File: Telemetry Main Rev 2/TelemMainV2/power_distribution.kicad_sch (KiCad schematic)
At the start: 8 parts, among them U1 LM7805_TO220, U2 LM7809_TO220

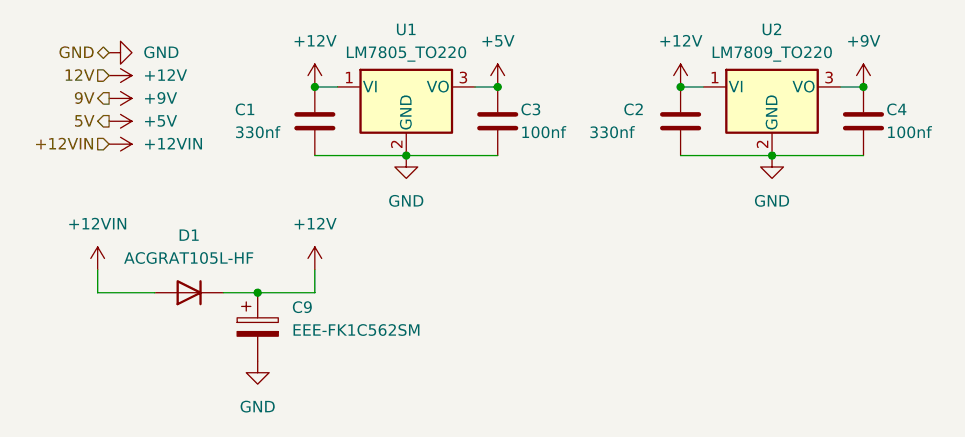
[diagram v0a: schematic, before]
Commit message: added status diodes, fixed silkscreen, etc
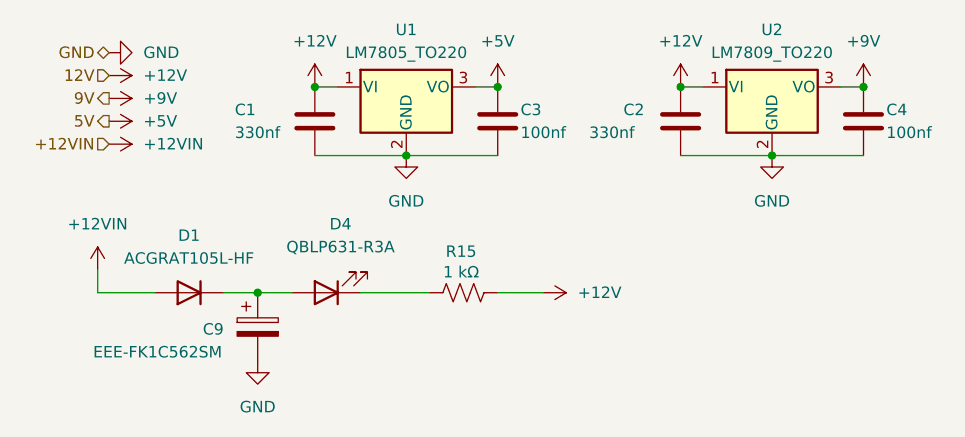
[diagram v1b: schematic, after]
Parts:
- added D4: QBLP631-R3A, LED_SMD:LED_0805_2012Metric_Pad1.15x1.40mm_HandSolder, symbol Device:LED
- added R15: 1 kΩ, Resistor_SMD:R_0805_2012Metric_Pad1.20x1.40mm_HandSolder, symbol Device:R_US
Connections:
- net +12V: now also R15.2; no longer C9.1, D1.1 (K)
- new net: D4.1 (K), R15.1
- new net: C9.1, D1.1 (K), D4.2 (A)
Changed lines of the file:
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@@
 	(wire
 		(pts
-			(xy 36.83 43.18) (xy 43.18 43.18)
+			(xy 36.83 43.18) (xy 40.64 43.18)
 		)
 		(stroke
@@
 	(wire
 		(pts
-			(xy 43.18 43.18) (xy 43.18 40.64)
+			(xy 48.26 43.18) (xy 55.88 43.18)
+		)
+		(stroke
+			(width 0)
+			(type default)
+		)
+	)
+	(wire
+		(pts
+			(xy 63.5 43.18) (xy 68.58 43.18)
 		)
 		(stroke
@@
 	)
 	(symbol
+		(lib_id "Device:LED")
+		(at 44.45 43.18 180)
+		(unit 1)
+		(exclude_from_sim no)
+		(in_bom yes)
+		(on_board yes)
+		(dnp no)
+		(fields_autoplaced yes)
+		(property "Reference" "D4"
+			(at 46.0375 35.56 0)
+			(effects
+				(font
+					(size 1.27 1.27)
+				)
+			)
+		)
+		(property "Value" "QBLP631-R3A"
+			(at 46.0375 38.1 0)
+			(effects
+				(font
+					(size 1.27 1.27)
+				)
+			)
+		)
+		(property "Footprint" "LED_SMD:LED_0805_2012Metric_Pad1.15x1.40mm_HandSolder"
+			(at 44.45 43.18 0)
+			(effects
+				(font
+					(size 1.27 1.27)
+				)
+				(hide yes)
+			)
+		)
+		(property "Datasheet" "https://www.qt-brightek.com/datasheet/QBLP631-R3A.pdf"
+			(at 44.45 43.18 0)
+			(effects
+				(font
+					(size 1.27 1.27)
+				)
+				(hide yes)
+			)
+		)
+		(property "Description" "12V Status LED"
+			(at 44.45 43.18 0)
+			(effects
+				(font
+					(size 1.27 1.27)
+				)
+				(hide yes)
+			)
+		)
+		(pin "1"
+		)
+		(pin "2"
+		)
+		(instances
+			(project "TelemMainV2"
+				(path "/dde73ecd-f7ea-407a-a1ab-cf1927044ecb/dcd9c4a0-8d80-4caa-a99a-0b76a5d913c0"
+					(reference "D4")
+					(unit 1)
+				)
+			)
+		)
+	)
+	(symbol
 		(lib_id "power:GND")
 		(at 20.32 16.51 90)
@@
 		(on_board yes)
 		(dnp no)
-		(fields_autoplaced yes)
 		(property "Reference" "C9"
-			(at 40.64 44.8309 0)
+			(at 30.734 47.244 0)
 			(effects
 				(font
@@
 		)
 		(property "Value" "EEE-FK1C562SM"
-			(at 40.64 47.3709 0)
+			(at 18.542 49.784 0)
 			(effects
 				(font
@@
 	(symbol
 		(lib_id "power:+12V")
-		(at 43.18 40.64 0)
+		(at 68.58 43.18 270)
 		(unit 1)
 		(exclude_from_sim no)
@@
 		(fields_autoplaced yes)
 		(property "Reference" "#PWR049"
-			(at 43.18 44.45 0)
+			(at 64.77 43.18 0)
 			(effects
 				(font
@@
 		)
 		(property "Value" "+12V"
-			(at 43.18 35.56 0)
-			(effects
-				(font
-					(size 1.27 1.27)
-				)
+			(at 72.39 43.1799 90)
+			(effects
+				(font
+					(size 1.27 1.27)
+				)
+				(justify left)
 			)
 		)
 		(property "Footprint" ""
-			(at 43.18 40.64 0)
+			(at 68.58 43.18 0)
 			(effects
 				(font
@@
 		)
 		(property "Datasheet" ""
-			(at 43.18 40.64 0)
+			(at 68.58 43.18 0)
 			(effects
 				(font
@@
 		)
 		(property "Description" "Power symbol creates a global label with name \"+12V\""
-			(at 43.18 40.64 0)
+			(at 68.58 43.18 0)
 			(effects
 				(font
@@
 					(unit 1)
 				)
+			)
+		)
+	)
+	(symbol
+		(lib_id "Device:R_US")
+		(at 59.69 43.18 90)
+		(unit 1)
+		(exclude_from_sim no)
+		(in_bom yes)
+		(on_board yes)
+		(dnp no)
+		(property "Reference" "R15"
+			(at 59.436 38.608 90)
+			(effects
+				(font
+					(size 1.27 1.27)
+				)
+			)
+		)
+		(property "Value" "1 kΩ"
+			(at 59.436 40.894 90)
+			(effects
+				(font
+					(size 1.27 1.27)
+				)
+			)
+		)
+		(property "Footprint" "Resistor_SMD:R_0805_2012Metric_Pad1.20x1.40mm_HandSolder"
+			(at 59.944 42.164 90)
+			(effects
+				(font
+					(size 1.27 1.27)
+				)
+				(hide yes)
+			)
+		)
+		(property "Datasheet" "~"
+			(at 59.69 43.18 0)
+			(effects
+				(font
+					(size 1.27 1.27)
+				)
+				(hide yes)
+			)
+		)
+		(property "Description" "Resistor, US symbol"
+			(at 59.69 43.18 0)
+			(effects
+				(font
+					(size 1.27 1.27)
+				)
+				(hide yes)
+			)
+		)
+		(pin "1"
+		)
+		(pin "2"
+		)
+		(instances
+			(project "TelemMainV2"
+				(path "/dde73ecd-f7ea-407a-a1ab-cf1927044ecb/dcd9c4a0-8d80-4caa-a99a-0b76a5d913c0"
+					(reference "R15")
+					(unit 1)
+				)
